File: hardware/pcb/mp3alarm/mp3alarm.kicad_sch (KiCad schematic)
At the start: 30 parts, among them IC1 RDA5807FP, J0 debug, J1 AUDIO, J10 Conn_Coaxial, J2 SW0, J3 SW1, J4 SW2, J5 I2C, J6 TM1637, J7 microSD, J8 5V, J9 ANT, U1 UDA1334A_Breakout, U2 mini_esp32, Y1 Crystal

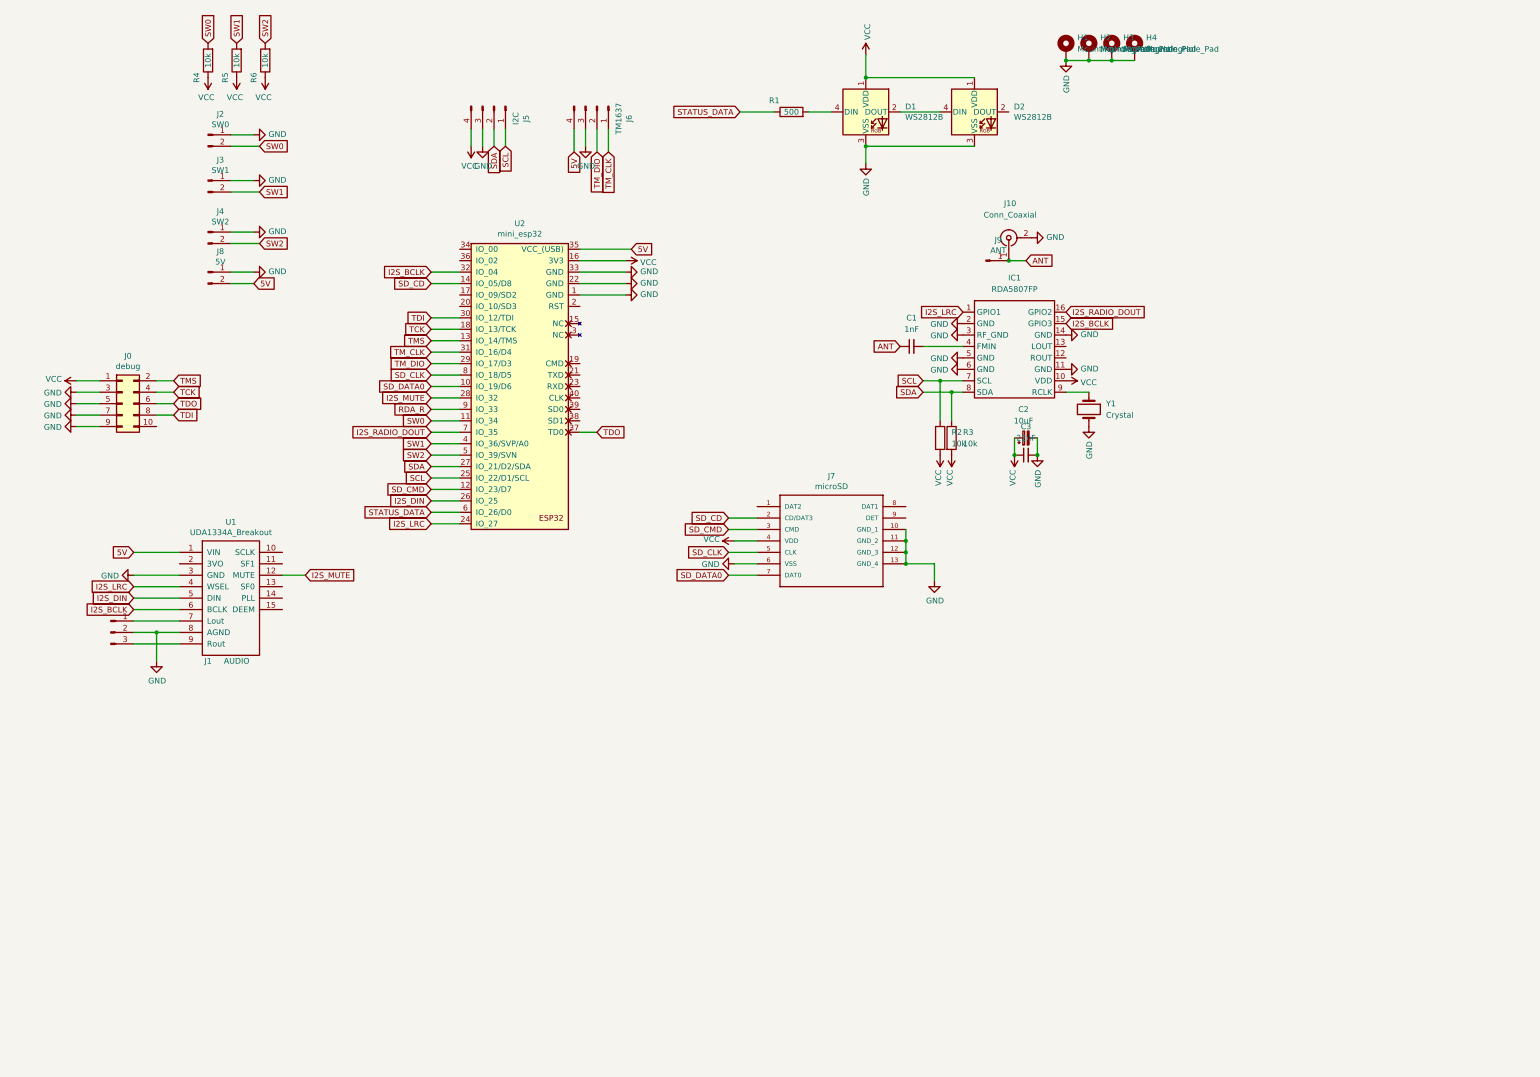
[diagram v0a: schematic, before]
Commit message: * Latest PCB update for ESP32S3
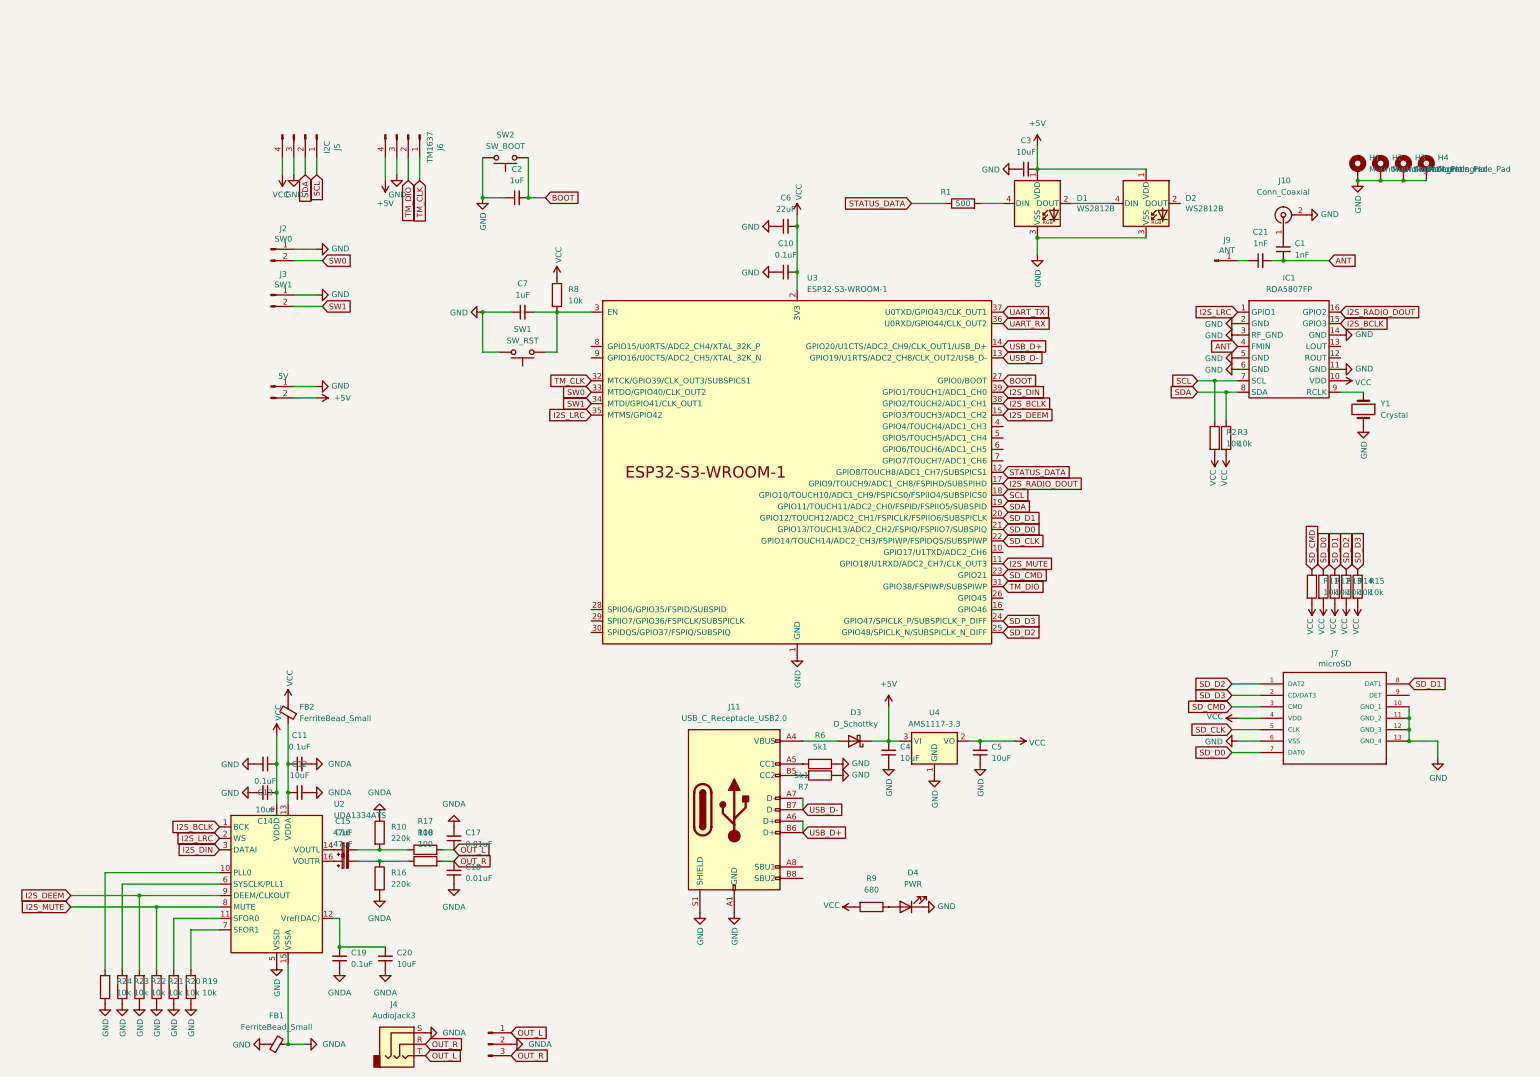
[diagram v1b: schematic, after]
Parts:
- removed C2: 10uF, Capacitor_SMD:C_Elec_6.3x5.4, symbol Device:C_Polarized_Small
- removed J0: debug, Connector_PinHeader_2.54mm:PinHeader_2x05_P2.54mm_Vertical_SMD, symbol Connector_Generic:Conn_02x05_Odd_Even
- removed J4: SW2, Connector_PinHeader_2.54mm:PinHeader_1x02_P2.54mm_Vertical, symbol Connector:Conn_01x02_Male
- removed R4, R5: 10k, Resistor_SMD:R_1206_3216Metric, symbol Device:R
- removed U1: UDA1334A_Breakout, UDA1334A:UDA1334A-breakout, symbol mp3alarm-rescue:UDA1334A_Breakout-UDA1334A
- removed U2: mini_esp32, pcb:ESP32_mini, symbol mp3alarm-rescue:mini_esp32-ESP32_mini
- added C10, C11, C13, C19: 0.1uF, Capacitor_SMD:C_1206_3216Metric, symbol Device:C_Small
- added C12, C14, C20, C4, C5: 10uF, Capacitor_SMD:C_1206_3216Metric, symbol Device:C_Small
- added C15, C16: 47uF, Capacitor_SMD:C_Elec_6.3x5.4, symbol Device:C_Polarized_Small
- added C17, C18: 0.01uF, Capacitor_SMD:C_1206_3216Metric, symbol Device:C_Small
- added C2, C7: 1uF, Capacitor_SMD:C_1206_3216Metric, symbol Device:C_Small
- added C21: 1nF, Capacitor_SMD:C_1206_3216Metric, symbol Device:C_Small
- added C6: 22uF, Capacitor_SMD:C_1206_3216Metric, symbol Device:C_Small
- added D3: D_Schottky, Diode_SMD:D_0805_2012Metric, symbol Device:D_Schottky
- added D4: PWR, LED_SMD:LED_0805_2012Metric, symbol Device:LED
- added FB1, FB2: FerriteBead_Small, Resistor_SMD:R_0805_2012Metric, symbol Device:FerriteBead_Small
- added J11: USB_C_Receptacle_USB2.0, Connector_USB:USB_C_Receptacle_JAE_DX07S016JA1R1500, symbol Connector:USB_C_Receptacle_USB2.0
- added J4: AudioJack3, footprints:PJ-313, symbol Connector_Audio:AudioJack3
- added R10, R16: 220k, Resistor_SMD:R_1206_3216Metric, symbol Device:R
- added R11, R12, R13, R14, R15, R19, R20, R21, R22, R23, R24, R8: 10k, Resistor_SMD:R_1206_3216Metric, symbol Device:R
- added R17, R18: 100, Resistor_SMD:R_1206_3216Metric, symbol Device:R
- added R7: 5k1, Resistor_SMD:R_1206_3216Metric, symbol Device:R
- added R9: 680, Resistor_SMD:R_1206_3216Metric, symbol Device:R
- added SW1: SW_RST, Button_Switch_SMD:SW_SPST_CK_RS282G05A3, symbol Switch:SW_Push
- added SW2: SW_BOOT, Button_Switch_SMD:SW_SPST_CK_RS282G05A3, symbol Switch:SW_Push
- added U2: UDA1334ATS, Package_SO:SSOP-16_4.4x5.2mm_P0.65mm, symbol Audio:UDA1334ATS
- added U3: ESP32-S3-WROOM-1, PCM_Espressif:ESP32-S3-WROOM-1, symbol PCM_Espressif:ESP32-S3-WROOM-1
- added U4: AMS1117-3.3, Package_TO_SOT_SMD:SOT-223-3_TabPin2, symbol Regulator_Linear:AMS1117-3.3
- C3: value 22nF -> 10uF
- R6: value 10k -> 5k1
- Y1: footprint Crystal:Crystal_C26-LF_D2.1mm_L6.5mm_Horizontal -> Crystal:Crystal_SMD_2012-2Pin_2.0x1.2mm
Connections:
- net ANT: now also IC1.4 (FMIN), C21.2; no longer J10.1 (In), J9.1 (Pin_1)
- net GND: now also C3.1, R6.1, C10.1, C13.2, C14.2, C2.1, C4.1, C5.1, C6.1, C7.1, D4.1 (K), FB1.1, J11.A1 (GND), J11.A12 (GND), J11.B1 (GND), J11.B12 (GND), J11.S1 (SHIELD), R19.1, R20.1, R21.1, R22.1, R23.1, R24.1, R7.1, SW1.2, SW2.2, U2.5 (VSSD), U3.1 (GND), U3.40 (GND), U3.41 (GND), U4.1 (GND); no longer C3.2, J1.2 (Pin_2)
- net I2S_BCLK: now also U2.1 (BCK), U3.38 (GPIO2/TOUCH2/ADC1_CH1)
- net I2S_DIN: now also U2.3 (DATAI), U3.39 (GPIO1/TOUCH1/ADC1_CH0)
- net I2S_LRC: now also U2.2 (WS), U3.35 (MTMS/GPIO42)
- net I2S_MUTE: now also R21.2, U2.8 (MUTE), U3.11 (GPIO18/U1RXD/ADC2_CH7/CLK_OUT3)
- net I2S_RADIO_DOUT: now also U3.17 (GPIO9/TOUCH9/ADC1_CH8/FSPIHD/SUBSPIHD)
- net SCL: now also U3.18 (GPIO10/TOUCH10/ADC1_CH9/FSPICS0/FSPIIO4/SUBSPICS0)
- net SDA: now also U3.19 (GPIO11/TOUCH11/ADC2_CH0/FSPID/FSPIIO5/SUBSPID)
- net SD_CLK: now also U3.22 (GPIO14/TOUCH14/ADC2_CH3/FSPIWP/FSPIDQS/SUBSPIWP)
- net SD_CMD: now also R11.1, U3.23 (GPIO21)
- net STATUS_DATA: now also U3.12 (GPIO8/TOUCH8/ADC1_CH7/SUBSPICS1)
- net SW0: now also U3.33 (MTDO/GPIO40/CLK_OUT2)
- net SW1: now also U3.34 (MTDI/GPIO41/CLK_OUT1)
- net TM_CLK: now also U3.32 (MTCK/GPIO39/CLK_OUT3/SUBSPICS1)
- net TM_DIO: now also U3.31 (GPIO38/FSPIWP/SUBSPIWP)
- net VCC: now also C10.2, C13.1, C14.1, C5.2, C6.2, FB2.2, R11.2, R12.2, R13.2, R14.2, R15.2, R8.1, R9.2, U2.4 (VDDD), U3.2 (3V3), U4.2 (VO); no longer C3.1, D1.1 (VDD), D2.1 (VDD), R6.1
- net OUT_L: now reaches J1.1 (Pin_1)
- net OUT_L: now also C17.1, J4.T, R17.2
- net OUT_R: now reaches J1.3 (Pin_3)
- net OUT_R: now also C18.2, J4.R, R18.2
- net SD_D2: now reaches J7.1 (DAT2)
- net SD_D2: now also R14.1, U3.25 (GPIO48/SPICLK_N/SUBSPICLK_N_DIFF)
- net SD_D1: now reaches J7.8 (DAT1)
- net SD_D1: now also R13.1, U3.20 (GPIO12/TOUCH12/ADC2_CH1/FSPICLK/FSPIIO6/SUBSPICLK)
- net at C1.2: now also J10.1 (In); no longer IC1.4 (FMIN)
- net 5V renamed +5V
- net +5V: now also C3.2, D1.1 (VDD), D2.1 (VDD), C4.2, D3.1 (K), U4.3 (VI)
- net SD_CD renamed SD_D3
- net SD_D3: now also R15.1, U3.24 (GPIO47/SPICLK_P/SUBSPICLK_P_DIFF)
- net SD_DATA0 renamed SD_D0
- net SD_D0: now also R12.1, U3.21 (GPIO13/TOUCH13/ADC2_CH2/FSPIQ/FSPIIO7/SUBSPIQ)
- net SW2: no longer names the net of R6.2
- net SW2: now also J11.A5 (CC1)
- new net: C21.1, J9.1 (Pin_1)
- new net: C7.2, R8.2, SW1.1, U3.3 (EN)
- new net: C11.1, C12.1, FB2.1, U2.13 (VDDA)
- new net: C15.1, U2.14 (VOUTL)
- new net: C15.2, R10.2, R17.1
- new net: R23.2, U2.6 (SYSCLK/PLL1)
- new net: C16.2, R16.1, R18.1
- new net: D3.2 (A), J11.A4 (VBUS), J11.A9 (VBUS), J11.B4 (VBUS), J11.B9 (VBUS)
- new net: R24.2, U2.10 (PLL0)
- new net: R20.2, U2.11 (SFOR0)
- new net: C19.2, C20.2, U2.12 (Vref(DAC))
- new net: C16.1, U2.16 (VOUTR)
- new net: R19.2, U2.7 (SFOR1)
- new net: D4.2 (A), R9.1
- new net: J11.B5 (CC2), R7.2
- new net BOOT: C2.2, SW2.1, U3.27 (GPIO0/BOOT)
- new net GNDA: C11.2, C12.2, C17.2, C18.1, C19.1, C20.1, FB1.2, J1.2 (Pin_2), J4.S, R10.1, R16.2, U2.15 (VSSA)
- new net I2S_DEEM: R22.2, U2.9 (DEEM/CLKOUT), U3.15 (GPIO3/TOUCH3/ADC1_CH2)
- new net UART_RX: U3.36 (U0RXD/GPIO44/CLK_OUT2)
- new net UART_TX: U3.37 (U0TXD/GPIO43/CLK_OUT1)
- new net USB_D+: J11.A6 (D+), J11.B6 (D+), U3.14 (GPIO20/U1CTS/ADC2_CH9/CLK_OUT1/USB_D+)
- new net USB_D-: J11.A7 (D-), J11.B7 (D-), U3.13 (GPIO19/U1RTS/ADC2_CH8/CLK_OUT2/USB_D-)
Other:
- moved on the sheet: C1, D1, D2, H1, H2, H3, H4, IC1, J10, J2, J3, J5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
